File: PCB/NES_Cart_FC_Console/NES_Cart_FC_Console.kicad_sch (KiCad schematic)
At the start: 2 parts, among them J1 Famicom_Cartridge, J2 F31L-1A7H1-11060

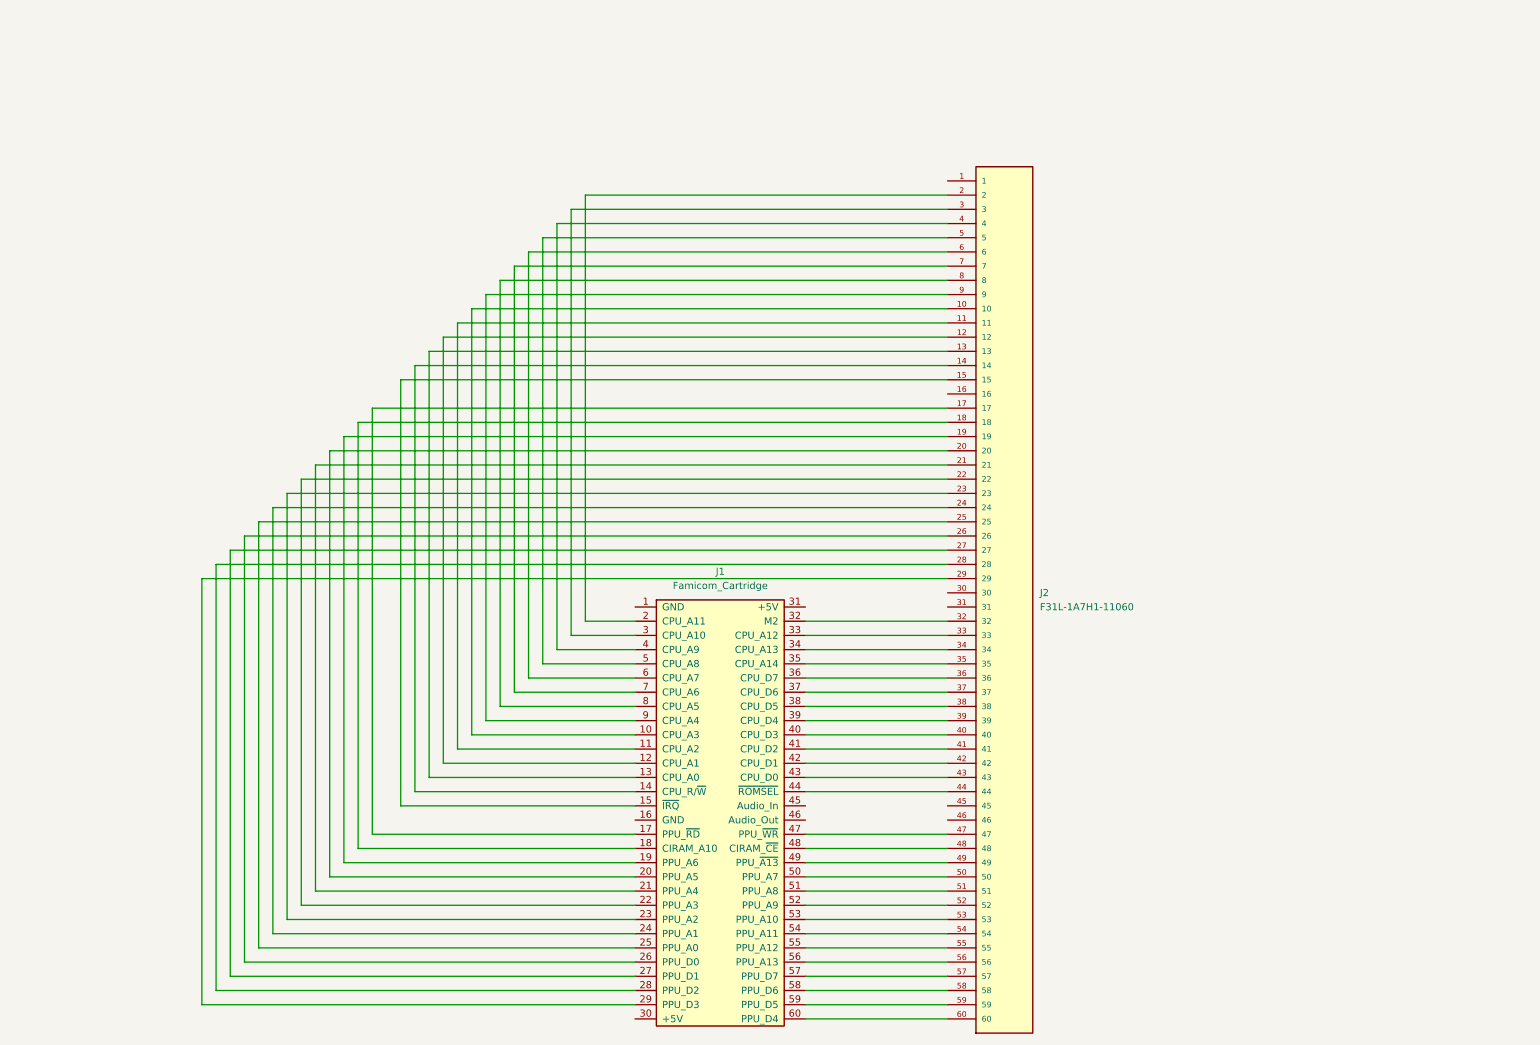
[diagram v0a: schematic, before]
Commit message: additional work done
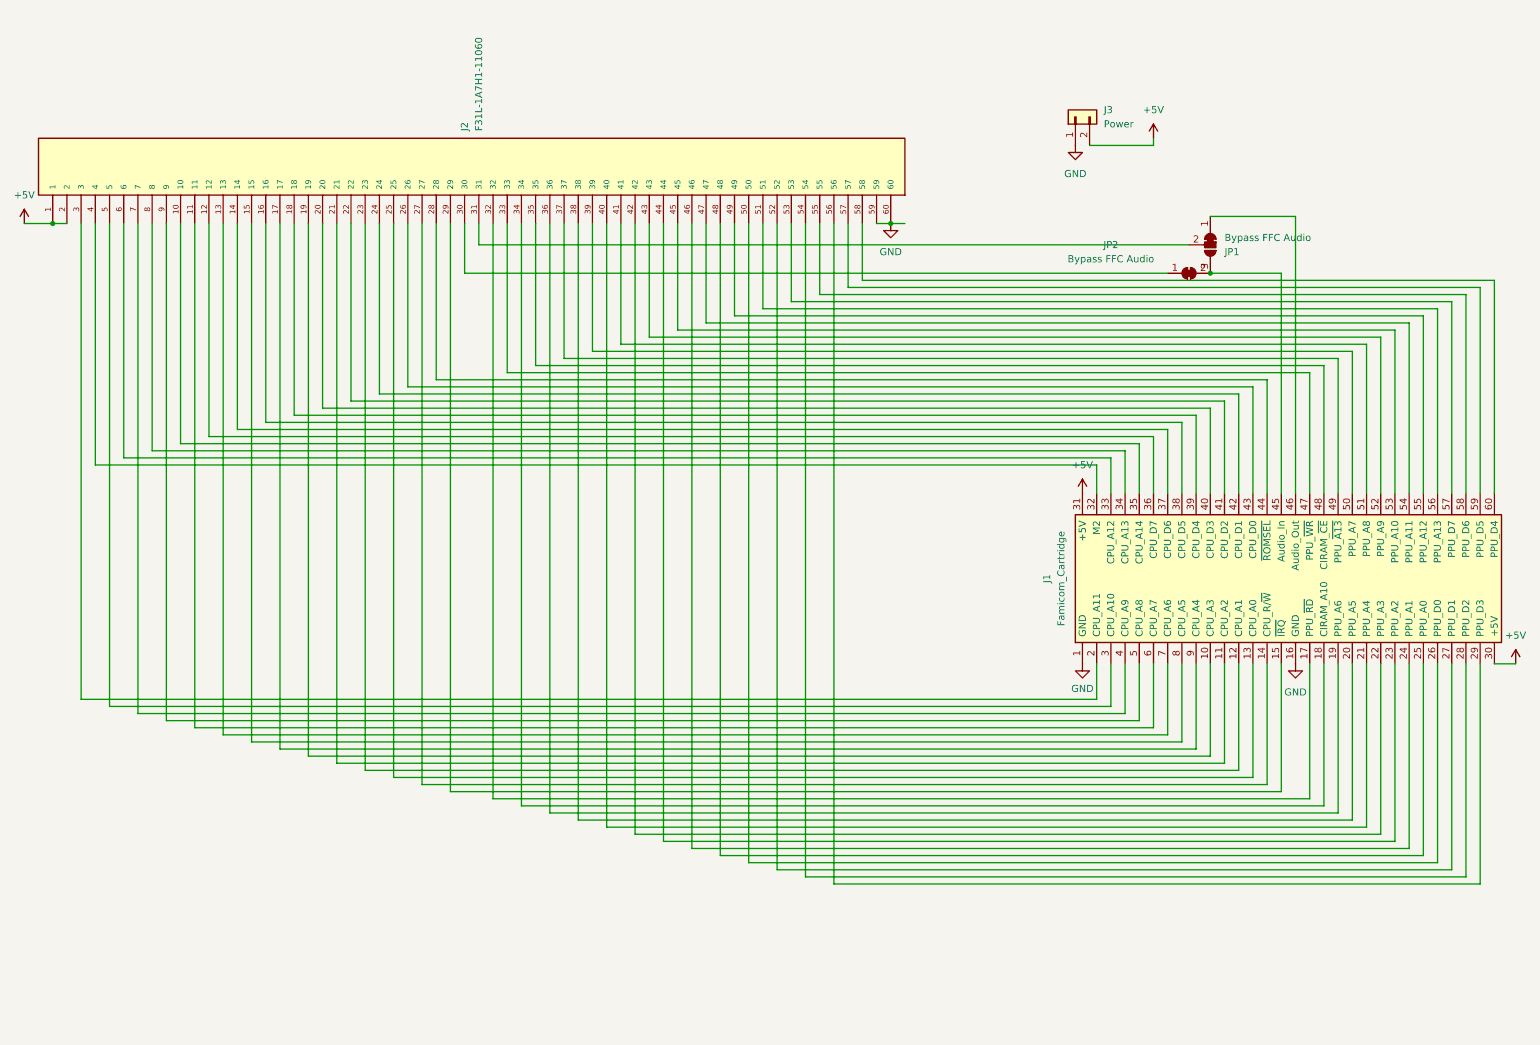
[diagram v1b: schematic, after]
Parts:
- added J3: Power, Connector_PinSocket_2.54mm:PinSocket_1x02_P2.54mm_Vertical, symbol Connector_Generic:Conn_01x02
- added JP1: Bypass FFC Audio, Jumper:SolderJumper-3_P1.3mm_Bridged2Bar12_RoundedPad1.0x1.5mm_NumberLabels, symbol Jumper:SolderJumper_3_Bridged12
- added JP2: Bypass FFC Audio, Jumper:SolderJumper-2_P1.3mm_Bridged_RoundedPad1.0x1.5mm, symbol Jumper:SolderJumper_2_Bridged
- J1: footprint (none) -> NES_Cart_FC_Console:Famicom_Card_Edge
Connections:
- net GND: now reaches J1.1 (GND)
- net GND: now also J1.16 (GND), J2.59, J2.60, J3.1 (Pin_1)
- net at J1.10 (CPU_A3): now also J2.19; no longer J2.10
- net at J1.11 (CPU_A2): now also J2.21; no longer J2.11
- net at J1.12 (CPU_A1): now also J2.23; no longer J2.12
- net at J1.13 (CPU_A0): now also J2.25; no longer J2.13
- net at J1.14 (CPU_R/~{W}): now also J2.27; no longer J2.14
- net at J1.15 (~{IRQ}): now also J2.29; no longer J2.15
- net at J1.17 (PPU_~{RD}): now also J2.32; no longer J2.17
- net at J1.18 (CIRAM_A10): now also J2.34; no longer J2.18
- net at J1.19 (PPU_A6): now also J2.36; no longer J2.19
- net at J1.2 (CPU_A11): now also J2.3; no longer J2.2
- net at J1.20 (PPU_A5): now also J2.38; no longer J2.20
- net at J1.21 (PPU_A4): now also J2.40; no longer J2.21
- net at J1.22 (PPU_A3): now also J2.42; no longer J2.22
- net at J1.23 (PPU_A2): now also J2.44; no longer J2.23
- net at J1.24 (PPU_A1): now also J2.46; no longer J2.24
- net at J1.25 (PPU_A0): now also J2.48; no longer J2.25
- net at J1.26 (PPU_D0): now also J2.50; no longer J2.26
- net at J1.27 (PPU_D1): now also J2.52; no longer J2.27
- net at J1.28 (PPU_D2): now also J2.54; no longer J2.28
- net at J1.29 (PPU_D3): now also J2.56; no longer J2.29
- net at J1.3 (CPU_A10): now also J2.5; no longer J2.3
- net +5V: now reaches J1.30 (+5V)
- net +5V: now also J1.31 (+5V), J2.1, J2.2, J3.2 (Pin_2)
- net at J1.32 (M2): now also J2.4; no longer J2.32
- net at J1.33 (CPU_A12): now also J2.6; no longer J2.33
- net at J1.34 (CPU_A13): now also J2.8; no longer J2.34
- net at J1.35 (CPU_A14): now also J2.10; no longer J2.35
- net at J1.36 (CPU_D7): now also J2.12; no longer J2.36
- net at J1.37 (CPU_D6): now also J2.14; no longer J2.37
- net at J1.38 (CPU_D5): now also J2.16; no longer J2.38
- net at J1.39 (CPU_D4): now also J2.18; no longer J2.39
- net at J1.4 (CPU_A9): now also J2.7; no longer J2.4
- net at J1.40 (CPU_D3): now also J2.20; no longer J2.40
- net at J1.41 (CPU_D2): now also J2.22; no longer J2.41
- net at J1.42 (CPU_D1): now also J2.24; no longer J2.42
- net at J1.43 (CPU_D0): now also J2.26; no longer J2.43
- net at J1.44 (~{ROMSEL}): now also J2.28; no longer J2.44
- net at J1.45 (Audio_In): now also JP1.3 (B), JP2.2 (B)
- net at J1.46 (Audio_Out): now also JP1.1 (A)
- net at J1.47 (PPU_~{WR}): now also J2.33; no longer J2.47
- net at J1.48 (CIRAM_~{CE}): now also J2.35; no longer J2.48
- net at J1.49 (PPU_~{A13}): now also J2.37; no longer J2.49
- net at J1.5 (CPU_A8): now also J2.9; no longer J2.5
- net at J1.50 (PPU_A7): now also J2.39; no longer J2.50
- net at J1.51 (PPU_A8): now also J2.41; no longer J2.51
- net at J1.52 (PPU_A9): now also J2.43; no longer J2.52
- net at J1.53 (PPU_A10): now also J2.45; no longer J2.53
- net at J1.54 (PPU_A11): now also J2.47; no longer J2.54
- net at J1.55 (PPU_A12): now also J2.49; no longer J2.55
- net at J1.56 (PPU_A13): now also J2.51; no longer J2.56
- net at J1.57 (PPU_D7): now also J2.53; no longer J2.57
- net at J1.58 (PPU_D6): now also J2.55; no longer J2.58
- net at J1.59 (PPU_D5): now also J2.57; no longer J2.59
- net at J1.6 (CPU_A7): now also J2.11; no longer J2.6
- net at J1.60 (PPU_D4): now also J2.58; no longer J2.60
- net at J1.7 (CPU_A6): now also J2.13; no longer J2.7
- net at J1.8 (CPU_A5): now also J2.15; no longer J2.8
- net at J1.9 (CPU_A4): now also J2.17; no longer J2.9
- net at J2.30: now also JP2.1 (A)
- net at J2.31: now also JP1.2 (C)
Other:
- moved on the sheet: J1, J2
